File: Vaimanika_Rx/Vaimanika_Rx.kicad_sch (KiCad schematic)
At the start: 53 parts, among them T1 0900PC16J0042001E, U1 LR1121IMLTRT, U2 RFX2401C, U3 SKY13373-460LF, U4 ESP32-C3FH4, U5 TLV75533PDQNR, U6 OW2EL89CENUXFMYLC-32M, U7 ANT3216LL00R2400A, U8 TS2306A 240GF MSM 9_C2976675, X1 CJ17-400001010B20

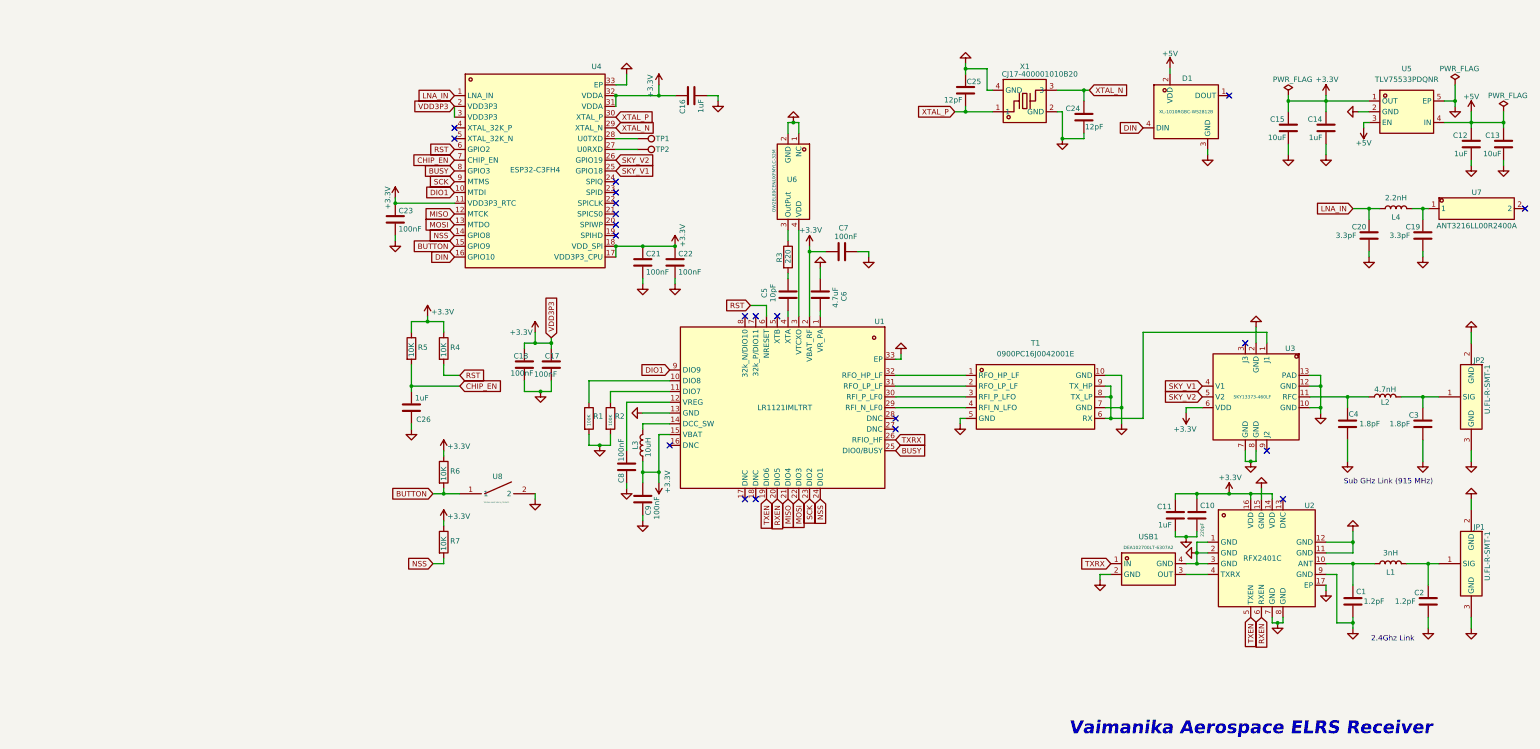
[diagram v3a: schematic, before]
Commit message: 25-05-2026
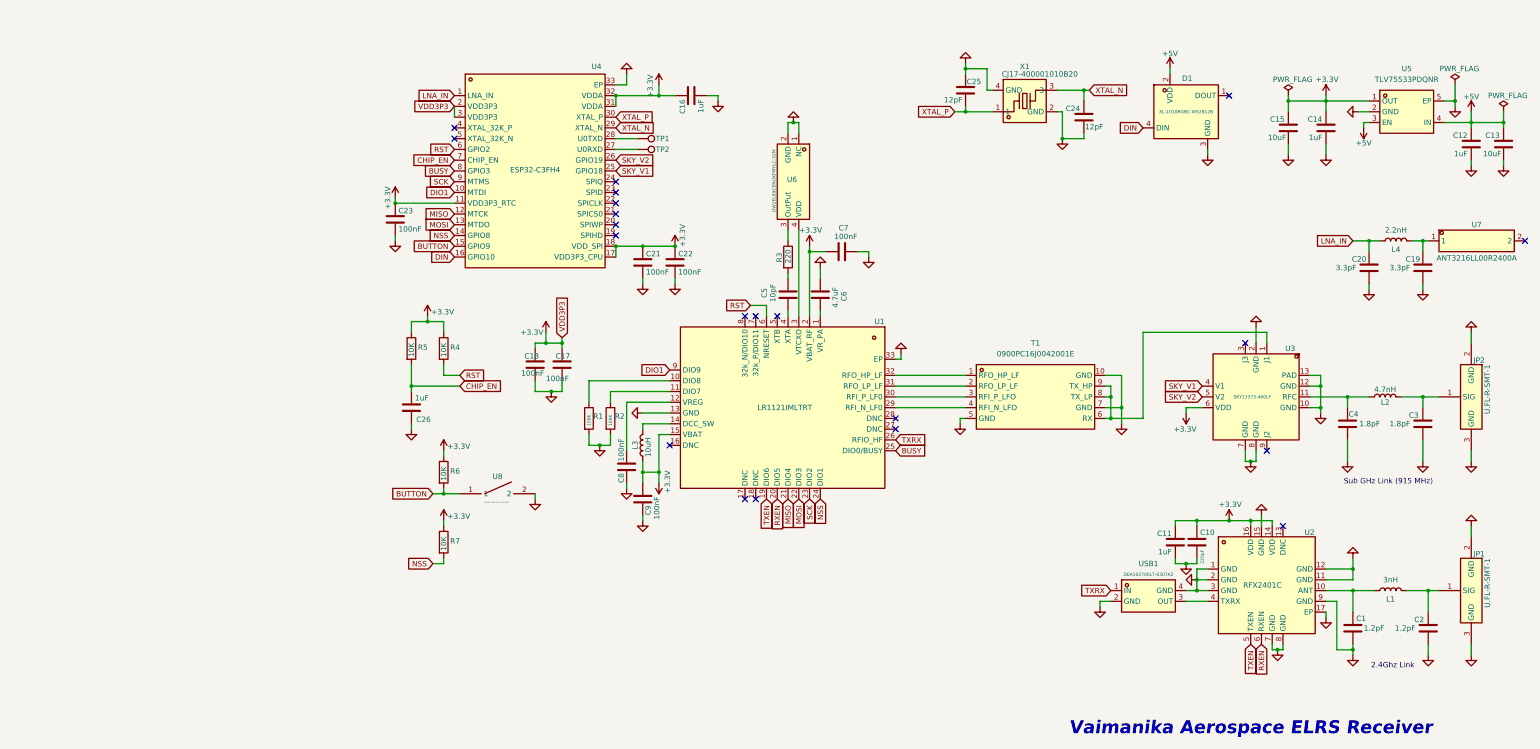
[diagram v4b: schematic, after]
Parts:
- U4: LCSC (none) -> C2858491; LCSC Part C2858491 -> (none)
- U5: LCSC (none) -> C2861882; LCSC Part C2861882 -> (none)
- U6: LCSC (none) -> C22434888; LCSC Part C22434888 -> (none)
- U7: LCSC (none) -> C293767; LCSC Part C293767 -> (none)
- U8: LCSC (none) -> C2976675; LCSC Part C2976675 -> (none)
- X1: LCSC (none) -> C2875272; LCSC Part C2875272 -> (none)
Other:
- moved on the sheet: C1, C10, C11, C17, C18, C19, C2, C20, JP1, L1, L4, U2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
